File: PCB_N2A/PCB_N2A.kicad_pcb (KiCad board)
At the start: 2 copper layers, 81 x 90 mm, 42 parts, among them J1 Conn_01x08, J2 Teclado, J3 LCD, J4 SENS, Q1 BC547, U1 68HC11_PLCC, U2 MAX232CPE, U3 24LC65, U4 MAX703, U5 DS1302+, U6 MAX491EPD, U7 DS1621, U8 24LC65, U9 EMI

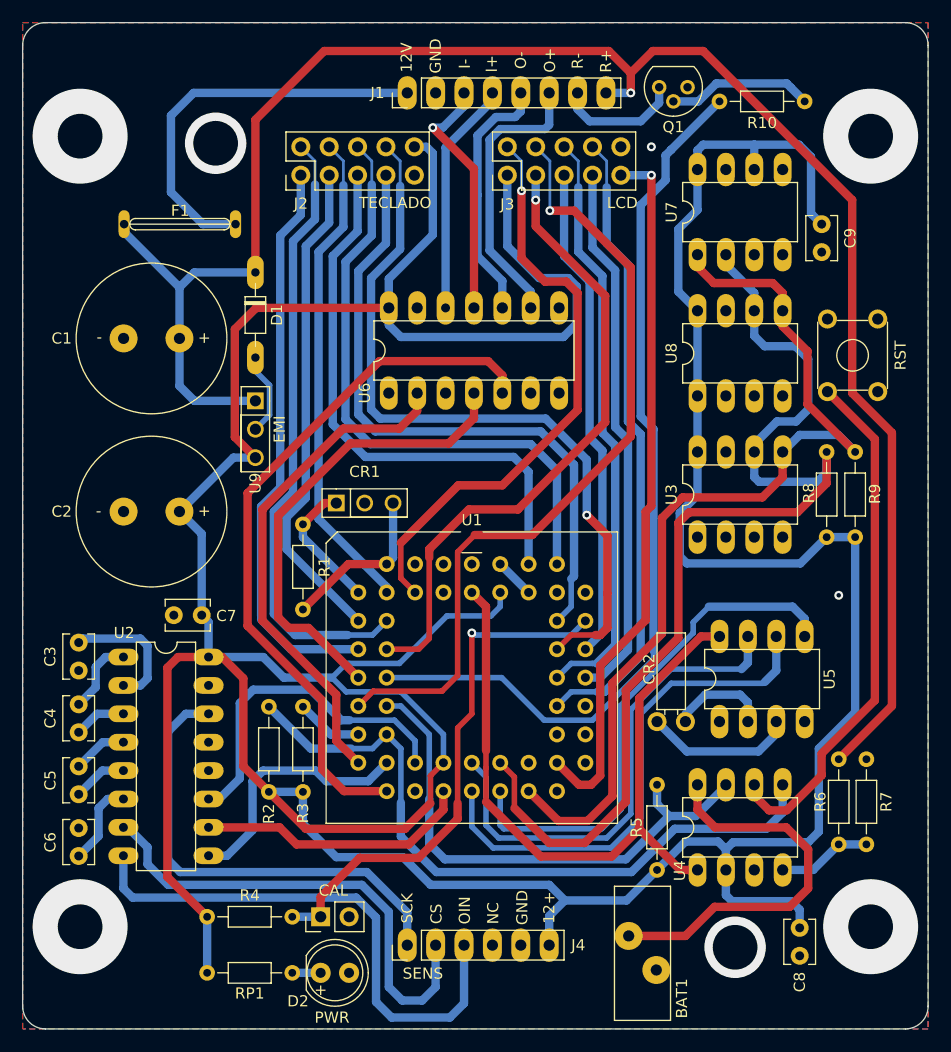
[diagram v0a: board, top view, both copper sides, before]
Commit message: wip
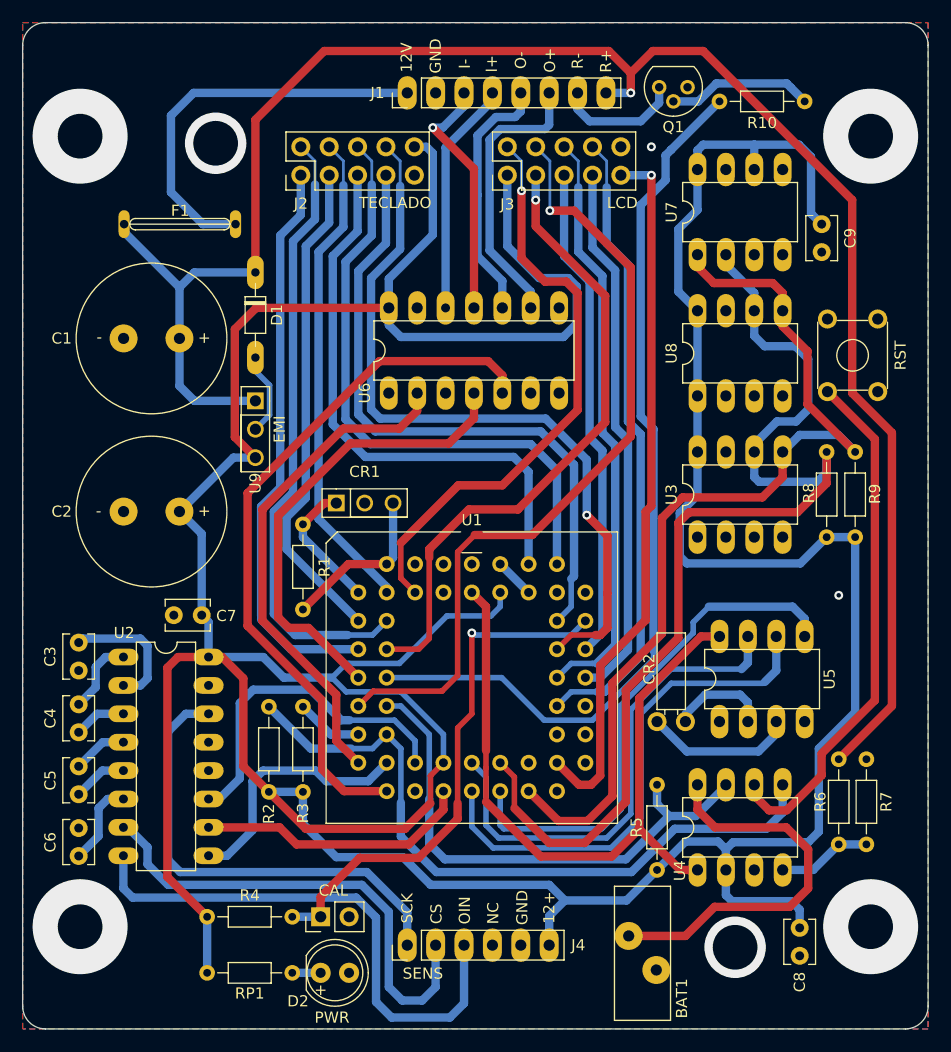
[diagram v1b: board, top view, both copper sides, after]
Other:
- net class Default removed
